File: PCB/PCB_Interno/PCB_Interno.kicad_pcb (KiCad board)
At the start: 2 copper layers, 81 x 81 mm, 5 parts, among them J2 Conn_02x24_Odd_Even

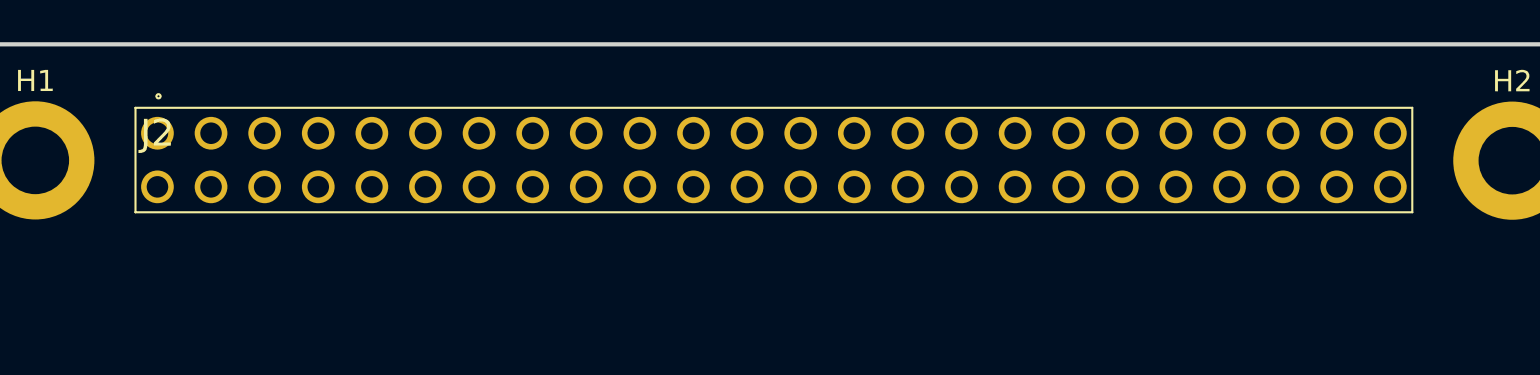
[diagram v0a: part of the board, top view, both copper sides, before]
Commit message: PC104
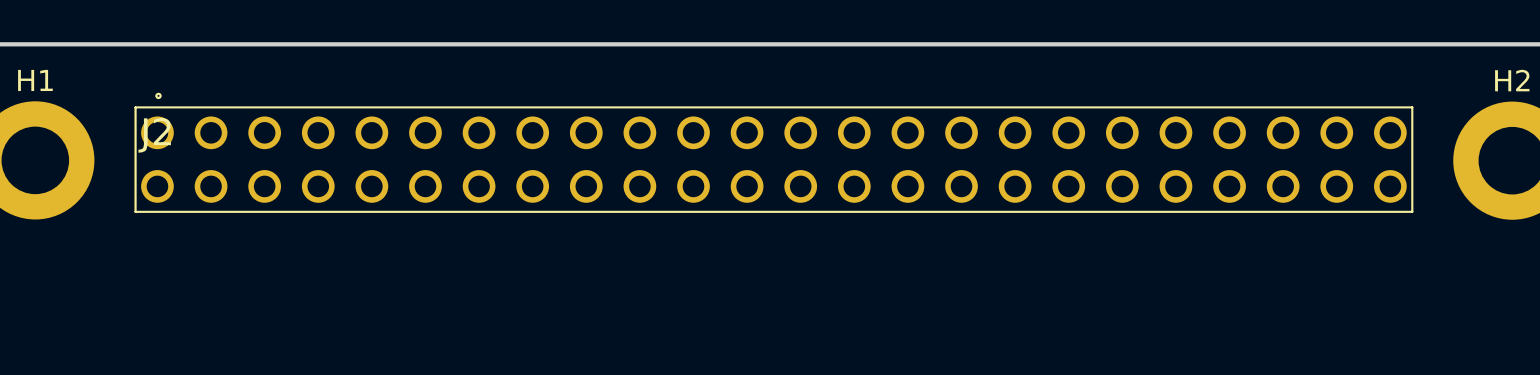
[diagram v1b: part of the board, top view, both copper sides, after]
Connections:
- net COMS_RX renamed ComsOBC_RX
- net COMS_TX renamed ObcComs_TX
- net Can_H renamed CAN_H
- net Can_L renamed CAN_L
- J2 pad 14: GND -> SW1
- J2 pad 15: SW2 -> EN_PY2
- J2 pad 16: SW1 -> SW2
- J2 pad 18: EN_PY2 -> EN_QUEMADOR
- J2 pad 2: +Vbatt -> NR
- J2 pad 27: I2C_SCL -> GND
- J2 pad 28: I2C_SDA -> GND
- J2 pad 29: GND -> I2C_SCL
- J2 pad 30: GND -> I2C_SDA
- J2 pad 40: GND -> CS_PY2
- J2 pad 41: unconnected-(J2-Pin_41-Pad41) -> CS_COMS
- J2 pad 43: unconnected-(J2-Pin_43-Pad43) -> SPI_MISO
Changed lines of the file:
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@@
 	(net 3 "I2C_SDA")
 	(net 4 "+Vbatt")
-	(net 5 "Can_L")
+	(net 5 "ComsOBC_RX")
 	(net 6 "SW2")
 	(net 7 "EN_ADCS")
@@
 	(net 10 "SPI_MOSI")
 	(net 11 "I2C_SCL")
-	(net 12 "Can_H")
+	(net 12 "CAN_L")
 	(net 13 "5V")
-	(net 14 "COMS_RX")
+	(net 14 "CAN_H")
 	(net 15 "EN_OBC")
 	(net 16 "PY2_RX")
@@
 	(net 19 "EN_PY2")
 	(net 20 "SPI_SCK")
-	(net 21 "COMS_TX")
+	(net 21 "ObcComs_TX")
 	(net 22 "EN_ADCS_5V")
-	(net 23 "unconnected-(J2-Pin_41-Pad41)")
-	(net 24 "unconnected-(J2-Pin_43-Pad43)")
+	(net 23 "CS_COMS")
+	(net 24 "NR")
+	(net 25 "SPI_MISO")
+	(net 26 "CS_PY2")
+	(net 27 "EN_QUEMADOR")
 	(footprint "MountingHole:MountingHole_3.2mm_M3_DIN965_Pad"
 		(layer "F.Cu")
@@
 	(footprint "KiCad:ESQ-124-Y-X-D"
 		(layer "F.Cu")
-		(at 167.8 55.2 180)
+		(at 167.8005 55.18 180)
 		(descr "ESQ-124-Y-X-D")
 		(tags "Connector")
@@
 			(layers "*.Cu" "*.Mask")
 			(remove_unused_layers no)
-			(net 4 "+Vbatt")
+			(net 24 "NR")
 			(pinfunction "Pin_2")
 			(pintype "passive")
@@
 			(layers "*.Cu" "*.Mask")
 			(remove_unused_layers no)
-			(net 1 "GND")
+			(net 9 "SW1")
 			(pinfunction "Pin_14")
 			(pintype "passive")
@@
 			(layers "*.Cu" "*.Mask")
 			(remove_unused_layers no)
-			(net 6 "SW2")
+			(net 19 "EN_PY2")
 			(pinfunction "Pin_15")
 			(pintype "passive")
@@
 			(layers "*.Cu" "*.Mask")
 			(remove_unused_layers no)
-			(net 9 "SW1")
+			(net 6 "SW2")
 			(pinfunction "Pin_16")
 			(pintype "passive")
@@
 			(layers "*.Cu" "*.Mask")
 			(remove_unused_layers no)
-			(net 19 "EN_PY2")
+			(net 27 "EN_QUEMADOR")
 			(pinfunction "Pin_18")
 			(pintype "passive")
@@
 			(layers "*.Cu" "*.Mask")
 			(remove_unused_layers no)
-			(net 12 "Can_H")
+			(net 14 "CAN_H")
 			(pinfunction "Pin_24")
 			(pintype "passive")
@@
 			(layers "*.Cu" "*.Mask")
 			(remove_unused_layers no)
-			(net 5 "Can_L")
+			(net 12 "CAN_L")
 			(pinfunction "Pin_26")
 			(pintype "passive")
@@
 			(layers "*.Cu" "*.Mask")
 			(remove_unused_layers no)
-			(net 11 "I2C_SCL")
+			(net 1 "GND")
 			(pinfunction "Pin_27")
 			(pintype "passive")
@@
 			(layers "*.Cu" "*.Mask")
 			(remove_unused_layers no)
-			(net 3 "I2C_SDA")
+			(net 1 "GND")
 			(pinfunction "Pin_28")
 			(pintype "passive")
@@
 			(layers "*.Cu" "*.Mask")
 			(remove_unused_layers no)
-			(net 1 "GND")
+			(net 11 "I2C_SCL")
 			(pinfunction "Pin_29")
 			(pintype "passive")
@@
 			(layers "*.Cu" "*.Mask")
 			(remove_unused_layers no)
-			(net 1 "GND")
+			(net 3 "I2C_SDA")
 			(pinfunction "Pin_30")
 			(pintype "passive")
@@
 			(layers "*.Cu" "*.Mask")
 			(remove_unused_layers no)
-			(net 1 "GND")
+			(net 26 "CS_PY2")
 			(pinfunction "Pin_40")
 			(pintype "passive")
@@
 			(layers "*.Cu" "*.Mask")
 			(remove_unused_layers no)
-			(net 23 "unconnected-(J2-Pin_41-Pad41)")
+			(net 23 "CS_COMS")
 			(pinfunction "Pin_41")
 			(pintype "passive")
@@
 			(layers "*.Cu" "*.Mask")
 			(remove_unused_layers no)
-			(net 24 "unconnected-(J2-Pin_43-Pad43)")
+			(net 25 "SPI_MISO")
 			(pinfunction "Pin_43")
 			(pintype "passive")
@@
 			(layers "*.Cu" "*.Mask")
 			(remove_unused_layers no)
-			(net 21 "COMS_TX")
+			(net 21 "ObcComs_TX")
 			(pinfunction "Pin_47")
 			(pintype "passive")
@@
 			(layers "*.Cu" "*.Mask")
 			(remove_unused_layers no)
-			(net 14 "COMS_RX")
+			(net 5 "ComsOBC_RX")
 			(pinfunction "Pin_48")
 			(pintype "passive")
